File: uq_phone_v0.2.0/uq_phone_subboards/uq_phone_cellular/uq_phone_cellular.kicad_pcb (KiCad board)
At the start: 4 copper layers, 45 x 30.2 mm, 32 parts, among them J1 513382474, J2 513382474, J3 20279-001E-03, J4 20279-001E-03, J5 20279-001E-03, U1 WP SNAP-IN BASE_6000636

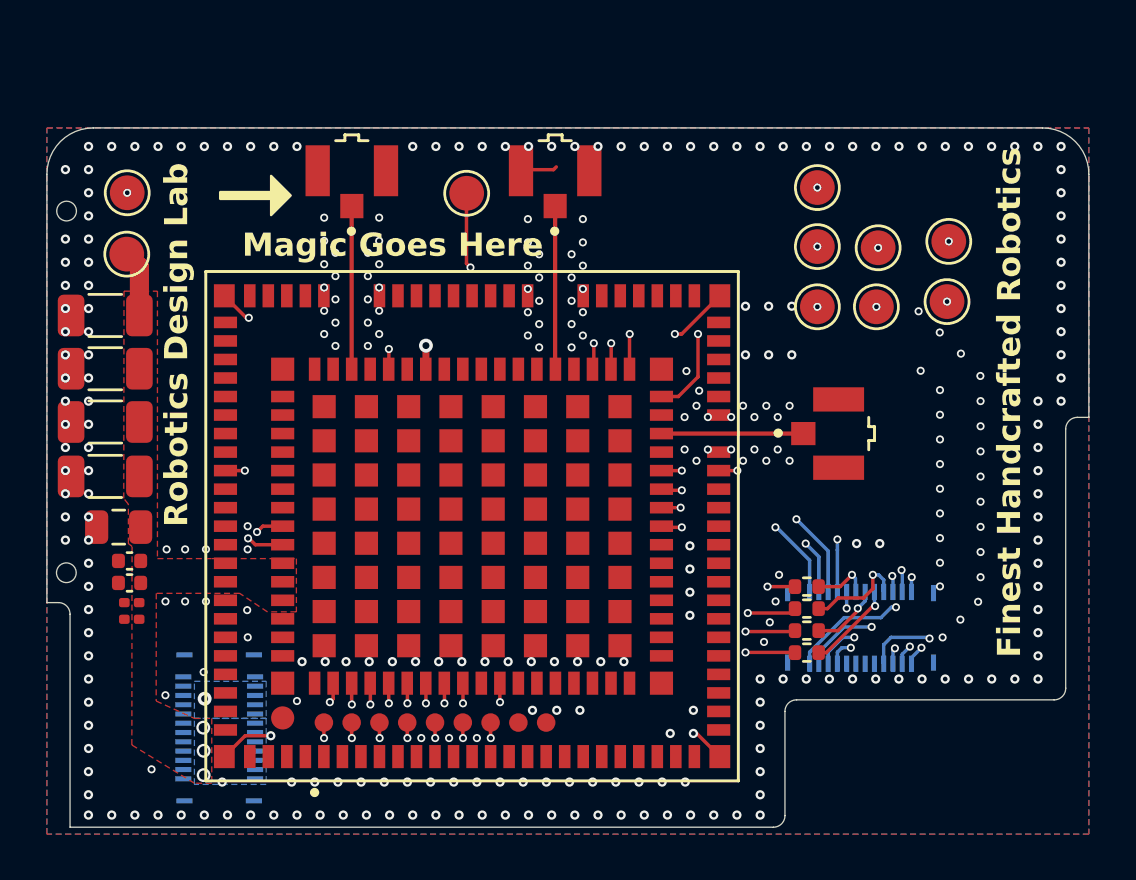
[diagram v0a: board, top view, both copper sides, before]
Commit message: Routing improvements
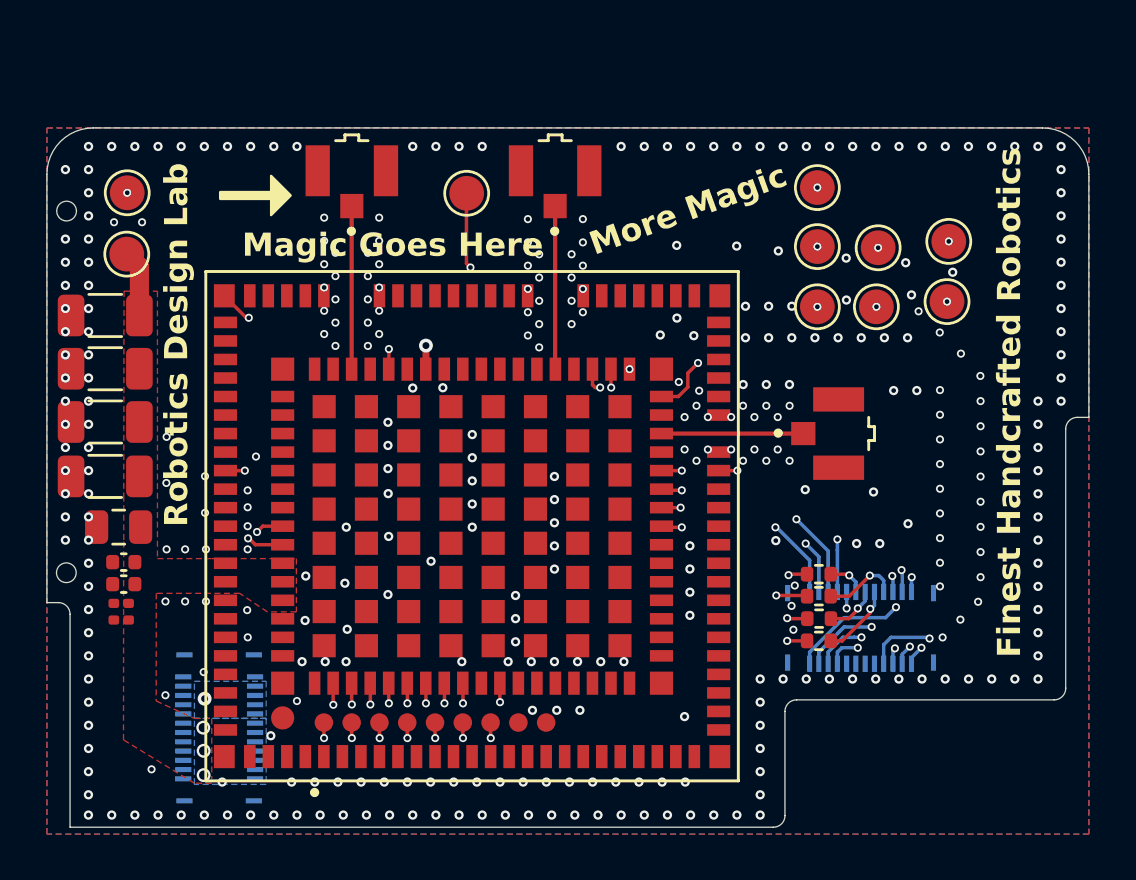
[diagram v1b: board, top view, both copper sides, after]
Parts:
- moved R3 0.75 mm to (101.9, 72.2)
- moved R1 0.75 mm to (101.9, 73.1)
- moved R4 0.74 mm to (102.0, 74.1)
- moved R2 0.73 mm to (101.9, 75.0)
- moved C3 0.46 mm to (71.8, 74.1)
- moved C4 0.46 mm to (71.8, 73.4)
- moved C1 0.26 mm to (71.9, 72.6)
- moved C2 0.26 mm to (71.9, 71.6)
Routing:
- net Net-(U1A-UART1_RX): track 29.4 -> 22.5 mm
- net GND: track 8.01 -> 1.45 mm, vias 318 -> 359
- net Net-(U1A-UART1_TX): track 29.0 -> 23.4 mm
- net Net-(U1A-UART1_CTS): track 28.7 -> 24.3 mm
- net Net-(U1A-UART1_RTS): track 28.4 -> 24.6 mm
- net MOB_RI: track 32.0 -> 29.2 mm
- net MOB_AUD_IN: track 33.6 -> 31.7 mm
- net MOB_PWR: track 43.5 -> 41.6 mm
- net MOB_AUD_OUT: track 32.4 -> 30.6 mm
- net MOB_SAFE_PWR_REMOVE_L: track 43.8 -> 42.1 mm
- net MOB_RST: track 24.9 -> 23.2 mm
- net (no net): track 1.42 -> 0.00 mm
- net Net-(U1A-J3): track 36.7 -> 35.5 mm
- net Net-(U1A-J5): track 38.0 -> 36.8 mm
- net Net-(U1A-J4): track 39.1 -> 38.0 mm
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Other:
- board text added: "More Magic"
